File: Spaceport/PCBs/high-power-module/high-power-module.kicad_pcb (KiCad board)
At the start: 4 copper layers, 37.4 x 37.6 mm, 83 parts, among them J1 Conn_01x06_Pin, J2 SMA, J3 Conn_01x06_Pin, J4 Conn_01x02_Pin, U1 Si4463, U2 SN74LV1T08QDBVRQ1, U3 TPS62177DQCR

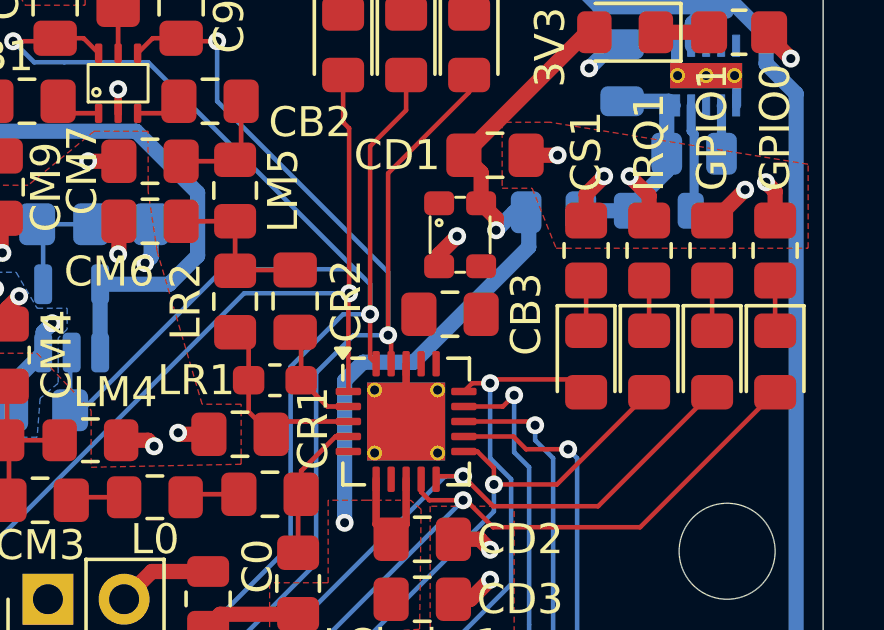
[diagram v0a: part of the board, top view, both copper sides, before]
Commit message: forgot to connect TCXO
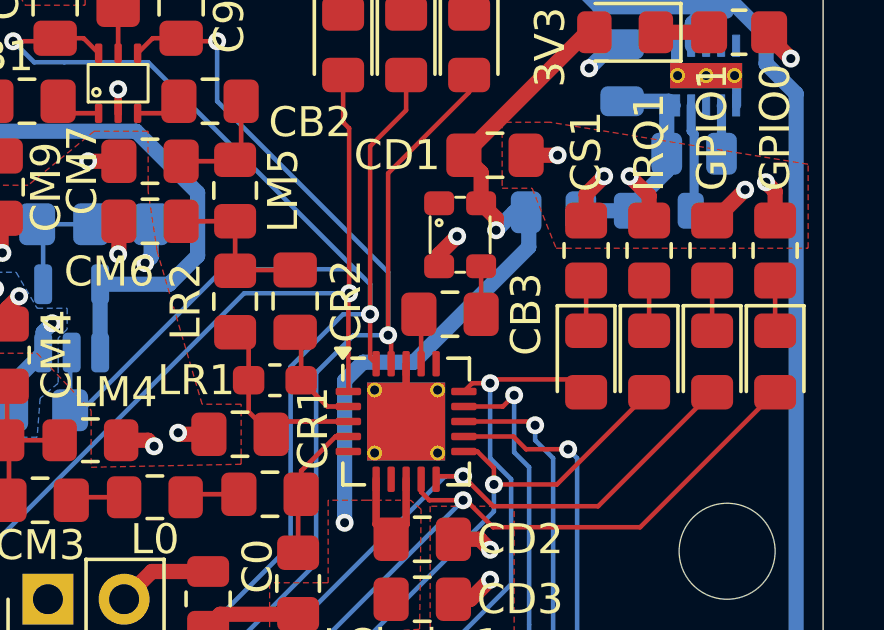
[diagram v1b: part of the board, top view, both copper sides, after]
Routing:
- net XO_IN: track 0.00 -> 1.68 mm
- net Net-(TCXO1-OUTPUT): track 0.00 -> 1.60 mm
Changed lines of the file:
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@@
 		(tags "capacitor handsolder")
 		(property "Reference" "CM6"
-			(at 1.3625 -1.68 360)
+			(at 1.3625 -1.68 0)
 			(layer "F.SilkS")
 			(effects
@@
 		)
 		(property "Value" "22pF"
-			(at 0 1.68 360)
+			(at 0 1.68 0)
 			(layer "F.Fab")
 			(hide yes)
@@
 		)
 		(fp_text user "${REFERENCE}"
-			(at 0 0 360)
+			(at 0 0 0)
 			(layer "F.Fab")
 			(effects
@@
 		(tags "inductor handsolder")
 		(property "Reference" "LM4"
-			(at -0.825 1.6 360)
+			(at -0.825 1.6 0)
 			(layer "F.SilkS")
 			(effects
@@
 		)
 		(property "Value" "18nH"
-			(at 0 1.65 360)
+			(at 0 1.65 0)
 			(layer "F.Fab")
 			(hide yes)
@@
 		)
 		(fp_text user "${REFERENCE}"
-			(at 0 0 360)
+			(at 0 0 0)
 			(layer "F.Fab")
 			(effects
@@
 		(tags "capacitor handsolder")
 		(property "Reference" "CM3"
-			(at 0 -1.5 360)
+			(at 0 -1.5 0)
 			(layer "F.SilkS")
 			(effects
@@
 		)
 		(property "Value" "6.2pF"
-			(at 0 1.68 360)
+			(at 0 1.68 0)
 			(layer "F.Fab")
 			(hide yes)
@@
 		)
 		(fp_text user "${REFERENCE}"
-			(at 0 0 360)
+			(at 0 0 0)
 			(layer "F.Fab")
 			(effects
@@
 		)
 		(property "Value" "22pF"
-			(at 0 1.68 360)
+			(at 0 1.68 0)
 			(layer "F.Fab")
 			(hide yes)
@@
 		)
 		(fp_text user "${REFERENCE}"
-			(at 0 0 360)
+			(at 0 0 0)
 			(layer "F.Fab")
 			(effects
@@
 		(tags "inductor handsolder")
 		(property "Reference" "L0"
-			(at 0 -1.4 360)
+			(at 0 -1.4 0)
 			(layer "F.SilkS")
 			(effects
@@
 		)
 		(property "Value" "15nH"
-			(at 0 1.65 360)
+			(at 0 1.65 0)
 			(layer "F.Fab")
 			(hide yes)
@@
 		)
 		(fp_text user "${REFERENCE}"
-			(at 0 0 360)
+			(at 0 0 0)
 			(layer "F.Fab")
 			(effects
@@
 		(tags "capacitor handsolder")
 		(property "Reference" "C2"
-			(at -2.7625 0 360)
+			(at -2.7625 0 0)
 			(layer "F.SilkS")
 			(effects
@@
 		)
 		(property "Value" "36pF"
-			(at 0 1.68 360)
+			(at 0 1.68 0)
 			(layer "F.Fab")
 			(hide yes)
@@
 		)
 		(fp_text user "${REFERENCE}"
-			(at 0 0 360)
+			(at 0 0 0)
 			(layer "F.Fab")
 			(effects
@@
 		(tags "capacitor handsolder")
 		(property "Reference" "CD3"
-			(at 3.2625 0 360)
+			(at 3.2625 0 0)
 			(layer "F.SilkS")
 			(effects
@@
 		)
 		(property "Value" "10uF"
-			(at 0 1.68 360)
+			(at 0 1.68 0)
 			(layer "F.Fab")
 			(hide yes)
@@
 		)
 		(fp_text user "${REFERENCE}"
-			(at 0 0 360)
+			(at 0 0 0)
 			(layer "F.Fab")
 			(effects
@@
 		(tags "capacitor handsolder")
 		(property "Reference" "CD2"
-			(at 3.2625 0 360)
+			(at 3.2625 0 0)
 			(layer "F.SilkS")
 			(effects
@@
 		)
 		(property "Value" "10uF"
-			(at 0 1.68 360)
+			(at 0 1.68 0)
 			(layer "F.Fab")
 			(hide yes)
@@
 		)
 		(fp_text user "${REFERENCE}"
-			(at 0 0 360)
+			(at 0 0 0)
 			(layer "F.Fab")
 			(effects
@@
 		(tags "capacitor handsolder")
 		(property "Reference" "CB2"
-			(at -3.3375 -0.7 360)
+			(at -3.3375 -0.7 0)
 			(layer "F.SilkS")
 			(effects
@@
 		)
 		(property "Value" "1uF"
-			(at 0 1.68 360)
+			(at 0 1.68 0)
 			(layer "F.Fab")
 			(hide yes)
@@
 		)
 		(fp_text user "${REFERENCE}"
-			(at 0 0 360)
+			(at 0 0 0)
 			(layer "F.Fab")
 			(effects
@@
 		)
 		(property "Value" "11nH"
-			(at 0 1.65 360)
+			(at 0 1.65 0)
 			(layer "F.Fab")
 			(hide yes)
@@
 		)
 		(fp_text user "${REFERENCE}"
-			(at 0 0 360)
+			(at 0 0 0)
 			(layer "F.Fab")
 			(effects
@@
 	)
 	(segment
+		(start 150.7 89.6)
+		(end 150.7 88)
+		(width 0.1524)
+		(layer "F.Cu")
+		(net 14)
+	)
+	(segment
+		(start 148.7 89.675)
+		(end 148.625 89.6)
+		(width 0.1524)
+		(layer "F.Cu")
+		(net 15)
+	)
+	(segment
+		(start 148.7 91.25)
+		(end 148.7 89.675)
+		(width 0.1524)
+		(layer "F.Cu")
+		(net 15)
+	)
+	(segment
